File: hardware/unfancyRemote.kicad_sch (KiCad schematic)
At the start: 42 parts, among them J1 Arduino Analog, J10 UART, J2 Arduino Digital, J3 HALL1, J4 HALL2, J5 PPM, J6 VIN, J7 VBAT, J8 Motor, J9 Extra analog 1, Q1 AO3401A, Q2 MMBT3904, Q3 MMBT3904, SW1 SW_Push, U1 E28-2G4M12S

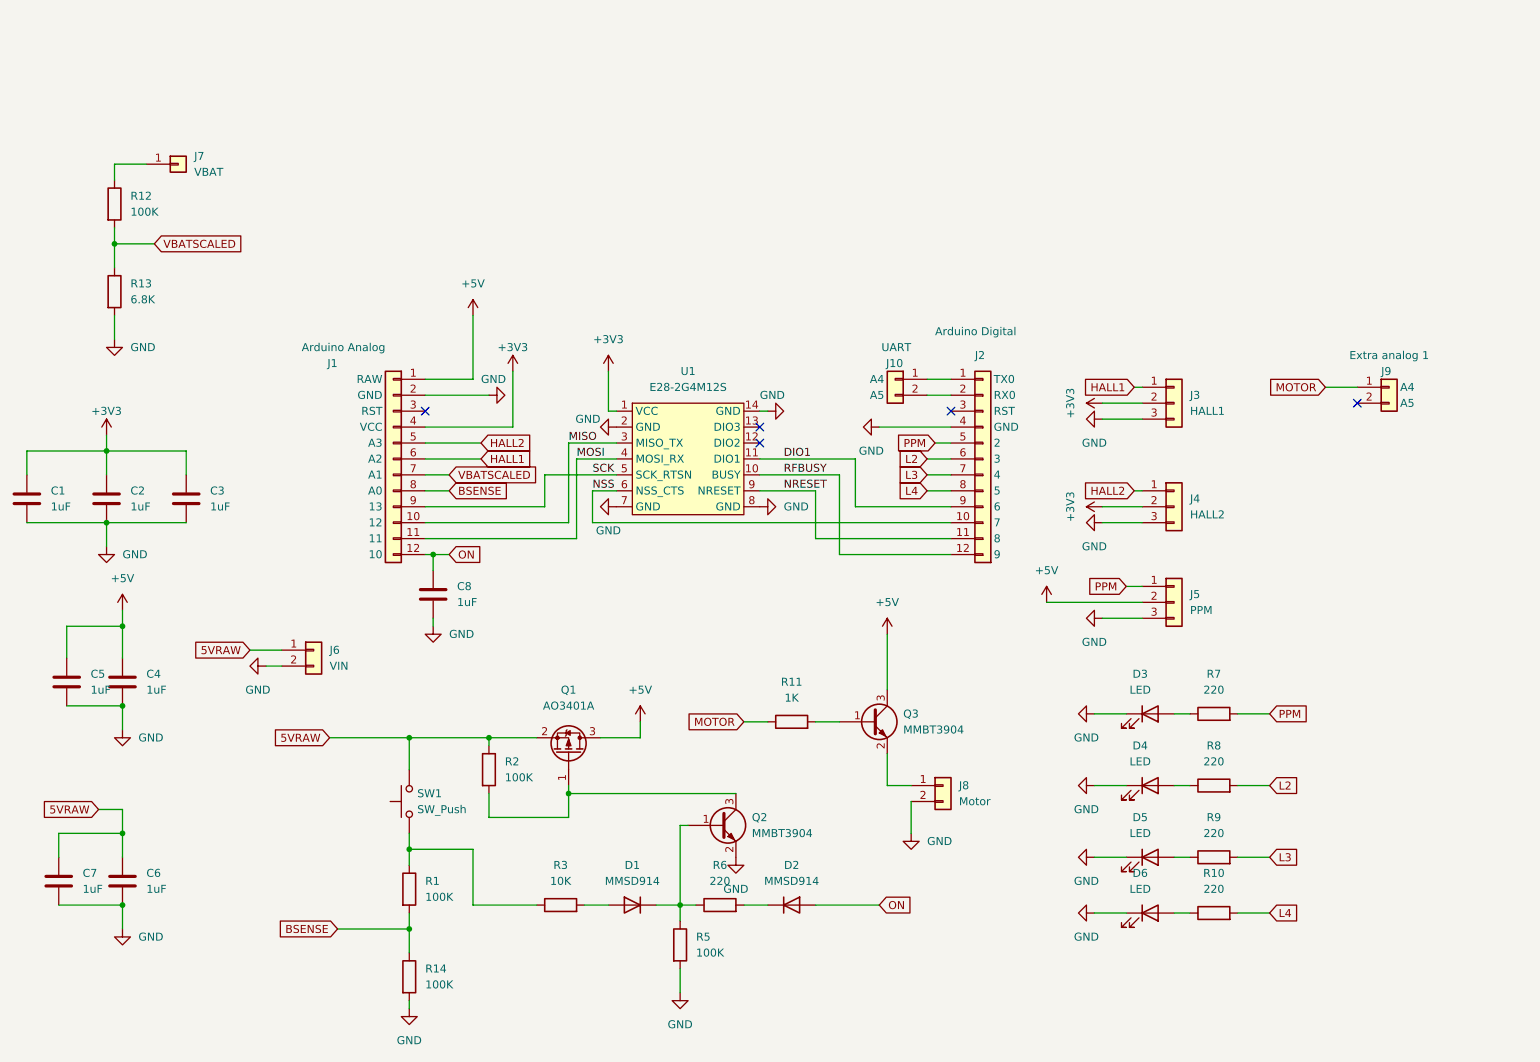
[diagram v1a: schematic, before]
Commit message: wip
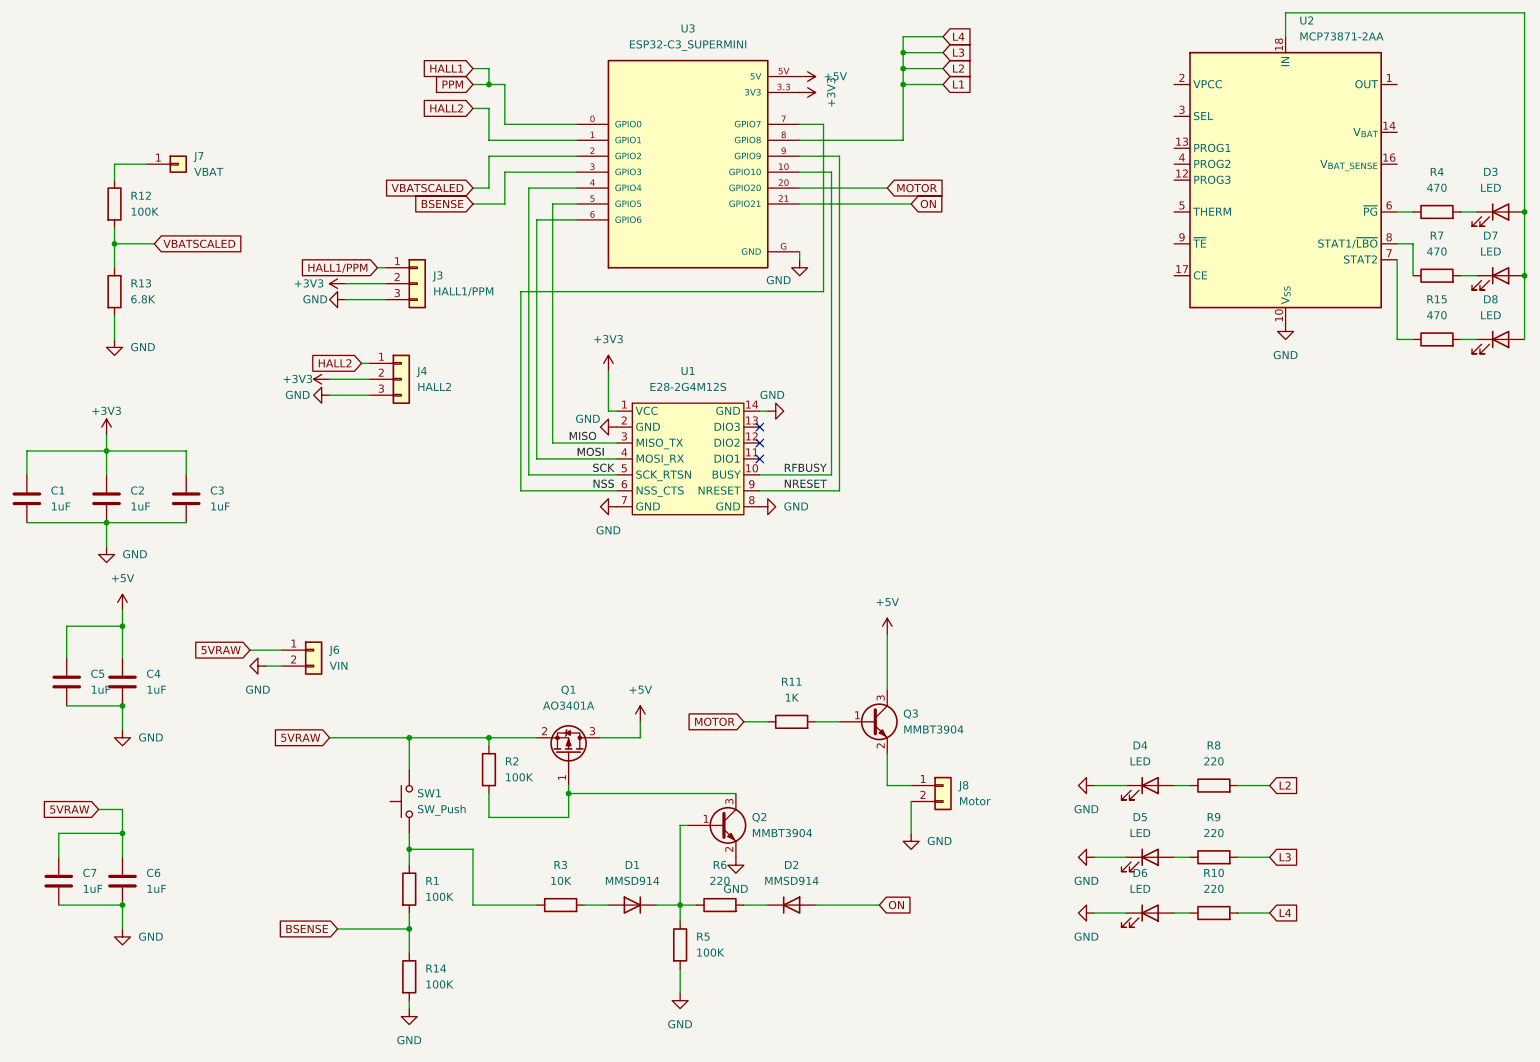
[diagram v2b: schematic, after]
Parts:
- removed C8: 1uF, Capacitor_SMD:C_0603_1608Metric, symbol Device:C
- removed J1: Arduino Analog, Connector_PinSocket_2.54mm:PinSocket_1x12_P2.54mm_Vertical, symbol unfancyRemote_components:Arduino_analog
- removed J10: UART, unfancyRemote_components:SolderWirePad_1x02_SMD_1x2mm, symbol unfancyRemote_components:Extra_analog_1
- removed J2: Arduino Digital, Connector_PinSocket_2.54mm:PinSocket_1x12_P2.54mm_Vertical, symbol unfancyRemote_components:Arduino_digital
- removed J5: PPM, unfancyRemote_components:SolderWirePad_1x03_SMD_1x2mm, symbol Connector_Generic:Conn_01x03
- removed J9: Extra analog 1, Connector_PinSocket_2.54mm:PinSocket_1x02_P2.54mm_Vertical, symbol unfancyRemote_components:Extra_analog_1
- added D7, D8: LED, LED_SMD:LED_0805_2012Metric, symbol Device:LED
- added R15, R4: 470, Resistor_SMD:R_0603_1608Metric, symbol Device:R
- added U2: MCP73871-2AA, Package_DFN_QFN:QFN-20-1EP_4x4mm_P0.5mm_EP2.5x2.5mm, symbol Battery_Management:MCP73871-2AA
- added U3: ESP32-C3_SUPERMINI, ESP32-C3_SUPERMINI:MODULE_ESP32-C3_SUPERMINI, symbol ESP32-C3_SUPERMINI:ESP32-C3_SUPERMINI
- J3: value HALL1 -> HALL1/PPM
- R7: value 220 -> 470
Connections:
- net L3 is gone; now on net L1: R9.2
- net L4 is gone; now on net L1: R10.2
- net +3V3: now also U3.3.3 (3V3)
- net +5V: now also U3.5V
- net BSENSE: now also U3.3 (GPIO3)
- net GND: now also U2.10 (V_{SS}), U2.11 (V_{SS}), U2.21 (V_{SS}), U3.G (GND); no longer D3.1 (K)
- net HALL1: now also U3.0 (GPIO0); no longer J3.1 (Pin_1)
- net HALL2: now also U3.1 (GPIO1)
- net MISO: now also U3.5 (GPIO5)
- net MOSI: now also U3.6 (GPIO6)
- net MOTOR: now also U3.20 (GPIO20)
- net NRESET: now also U3.9 (GPIO9)
- net NSS: now also U3.7 (GPIO7)
- net ON: now also U3.21 (GPIO21)
- net RFBUSY: now also U3.10 (GPIO10)
- net SCK: now also U3.4 (GPIO4)
- net VBATSCALED: now also U3.2 (GPIO2)
- net at D3.2 (A): now also D7.2 (A), D8.2 (A), U2.18 (IN), U2.19 (IN); no longer R7.1
- net DIO1: no longer names the net of U1.11 (DIO1)
- net L2 renamed L1
- net L1: now also U3.8 (GPIO8)
- net PPM: no longer names the net of R7.2
- net PPM: now also D7.1 (K)
- new net: D8.1 (K), R15.2
- new net: R7.1, U2.8 (STAT1/~{LBO})
- new net: R15.1, U2.7 (STAT2)
- new net: U2.1 (OUT), U2.20 (OUT)
- new net: U2.14 (V_{BAT}), U2.15 (V_{BAT})
- new net: R4.1, U2.6 (~{PG})
- new net: D3.1 (K), R4.2
- new net HALL1/PPM: J3.1 (Pin_1)
- no-connect marks 5 -> 3
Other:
- moved on the sheet: J3, J4
